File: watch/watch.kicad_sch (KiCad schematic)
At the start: 37 parts, among them IC1 MAX77659AENV+, J1 TYPE-C-31-M-12, J2 Conn_01x02_Socket, J3 Conn_ARM_JTAG_SWD_10, SW1 SW_Push, U1 nRF52840, Y1 32MHz

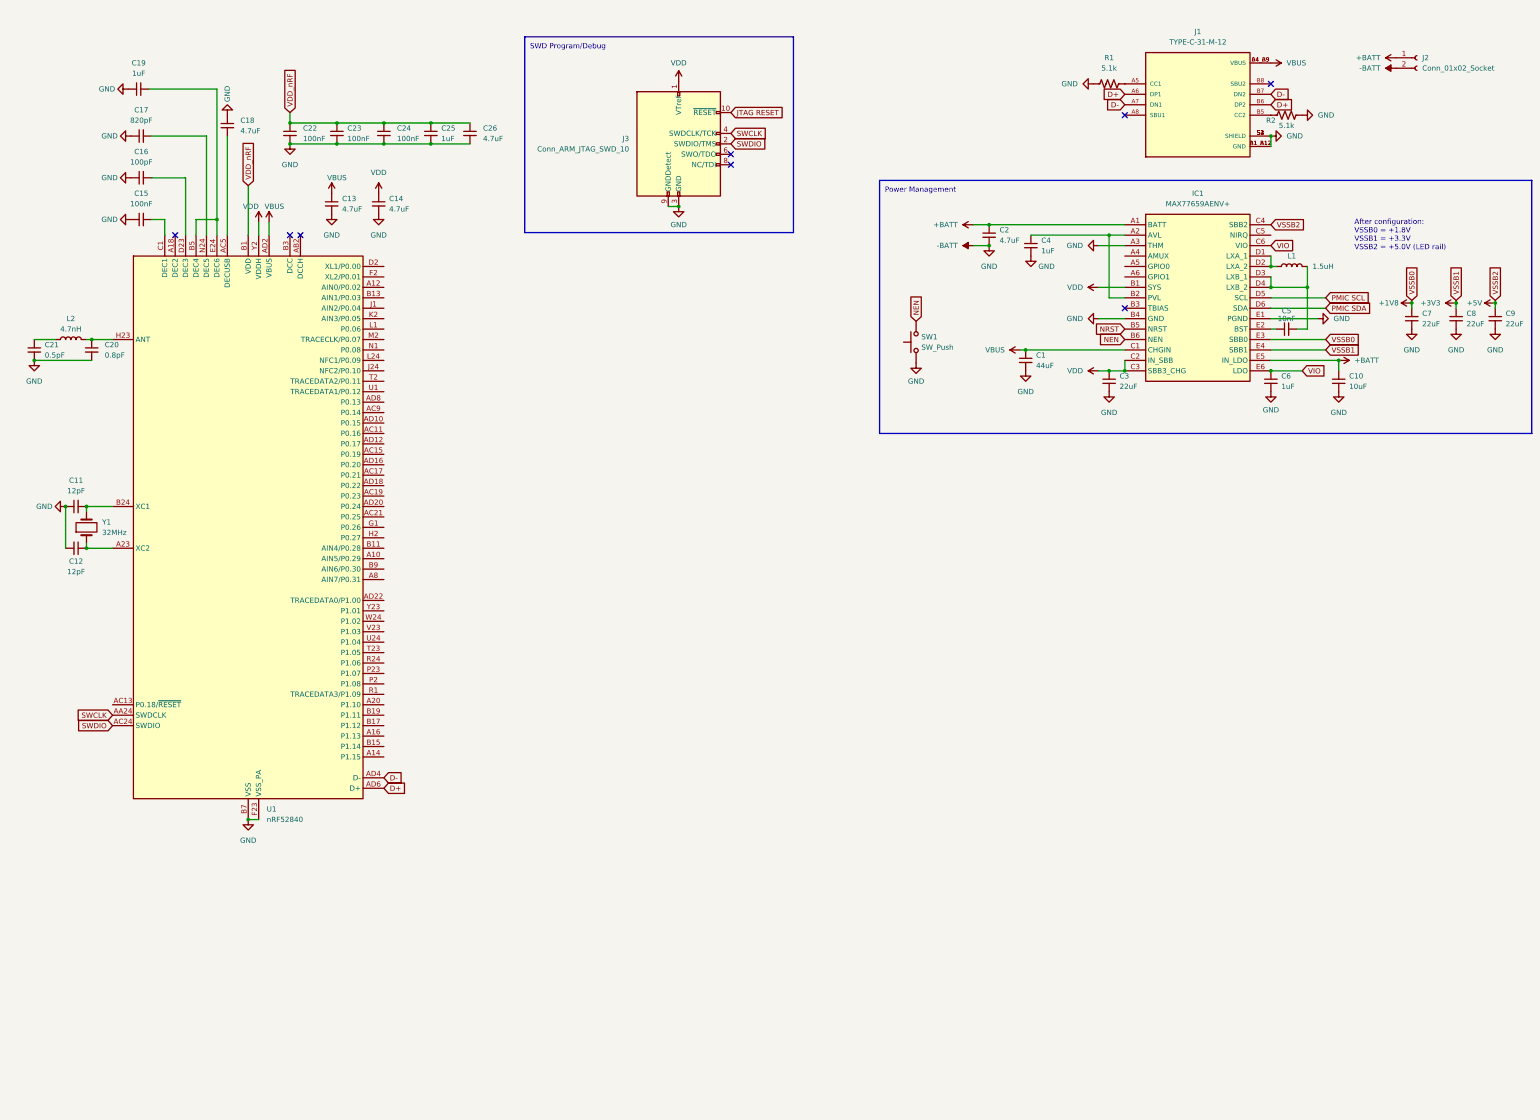
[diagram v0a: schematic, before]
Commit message: organize and add display block, going to the gym
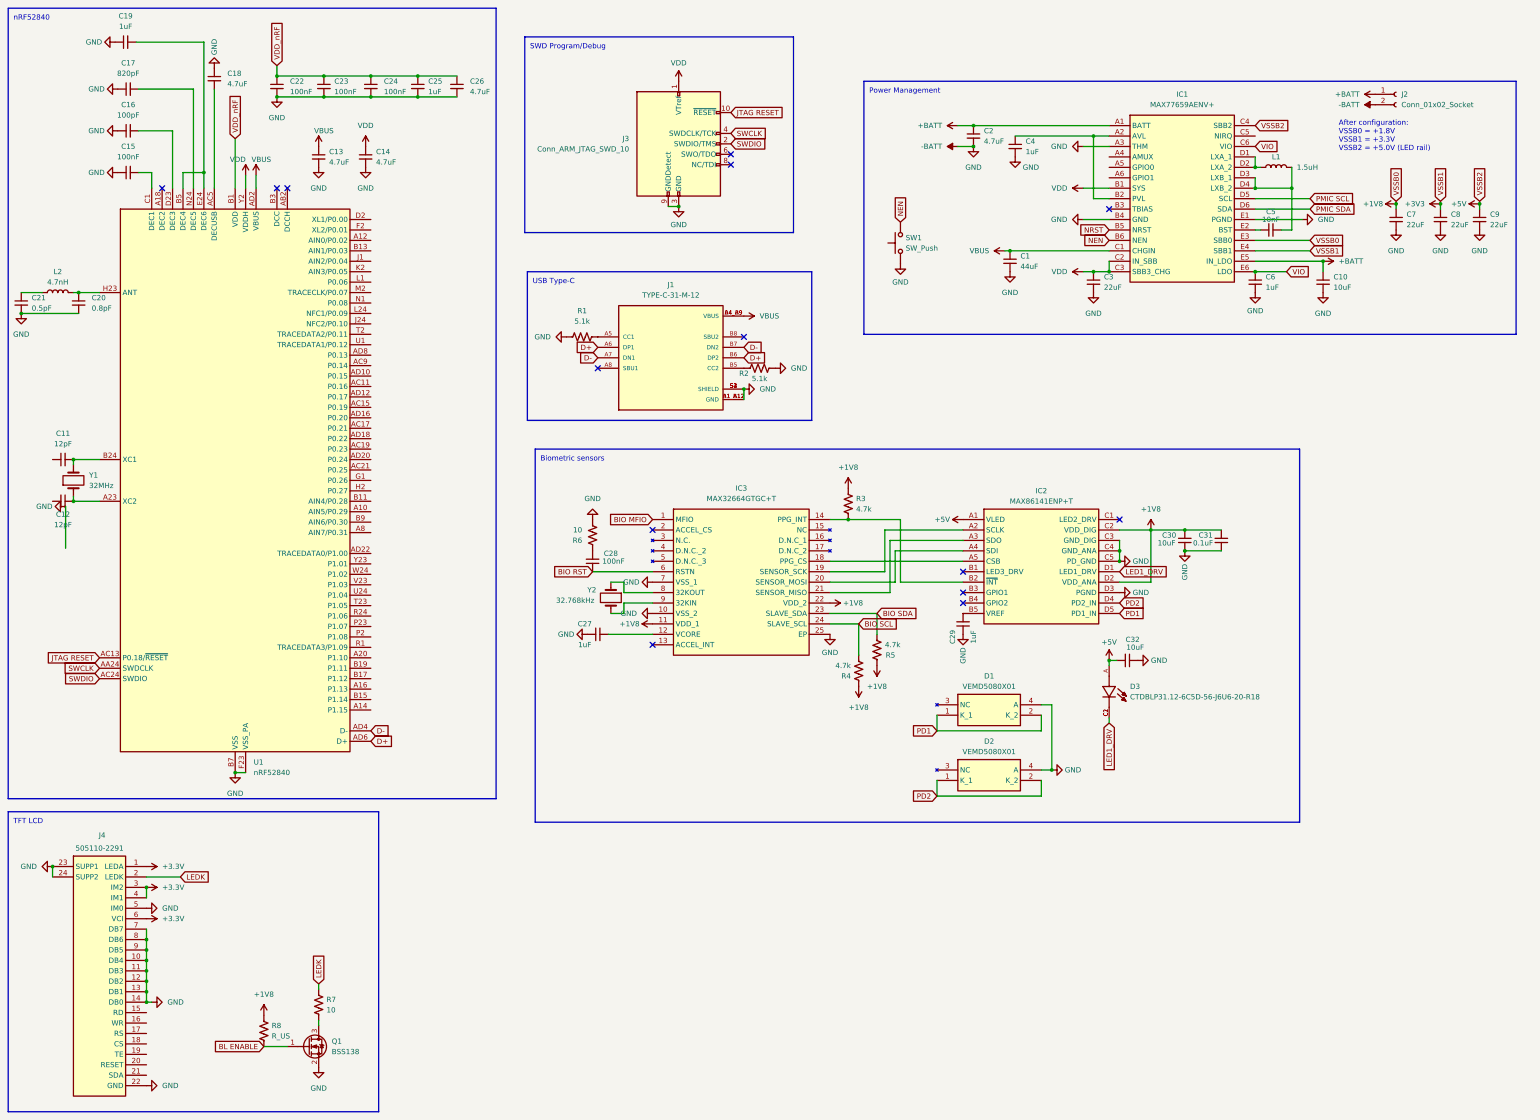
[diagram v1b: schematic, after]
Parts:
- added C27, C29: 1uF, symbol Device:C_Small
- added C28: 100nF, symbol Device:C_Small
- added C30, C32: 10uF, symbol Device:C_Small
- added C31: 0.1uF, symbol Device:C_Small
- added D1, D2: VEMD5080X01, VEMD5080X01, symbol VEMD5080X01:VEMD5080X01
- added D3: CTDBLP31.12-6C5D-56-J6U6-20-R18, LED_CTDBLP31.12-6C5D-56-J6U6-20-R18, symbol CTDBLP31.12-6C5D-56-J6U6-20-R18:CTDBLP31.12-6C5D-56-J6U6-20-R18
- added IC2: MAX86141ENP+T, BGA20C40P5X4_205X185X50, symbol MAX86141ENP+T:MAX86141ENP+T
- added IC3: MAX32664GTGC+T, MAX32664GTGC, symbol MAX32664GTGC+T:MAX32664GTGC+T
- added J4: 505110-2291, 5051102291, symbol 505110-2291:505110-2291
- added Q1: BSS138, Package_TO_SOT_SMD:SOT-23, symbol Transistor_FET:BSS138
- added R3, R4, R5: 4.7k, symbol Device:R_US
- added R6, R7: 10, symbol Device:R_US
- added R8: R_US, symbol Device:R_US
- added Y2: 32.768kHz, symbol Device:Crystal
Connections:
- net +1V8: now also C30.2, C31.2, IC2.C2 (VDD_DIG), IC2.D2 (VDD_ANA), IC3.11 (VDD_1), IC3.22 (VDD_2), R3.1, R4.1, R5.1, R8.1
- net +5V: now also C32.2, D3.A, IC2.A1 (VLED)
- net -BATT: now also C27.1, C29.1, C30.1, C31.1, C32.1, D1.4 (A), D2.4 (A), IC2.C3 (GND_DIG), IC2.C4 (GND_ANA), IC2.C5 (PD_GND), IC2.D3 (PGND), IC3.10 (VSS_2), IC3.25 (EP), IC3.7 (VSS_1), J4.10 (DB4), J4.11 (DB3), J4.12 (DB2), J4.13 (DB1), J4.14 (DB0), J4.22 (GND), J4.23 (SUPP1), J4.24 (SUPP2), J4.5 (IM0), J4.7 (DB7), J4.8 (DB6), J4.9 (DB5), Q1.2 (S), R6.1; no longer C11.1, C12.2
- net JTAG RESET: now also U1.AC13 (P0.18/~{RESET})
- new net: Q1.3 (D), R7.2
- new net: C28.2, R6.2
- new net: IC3.8 (32KOUT), Y2.1
- new net: IC3.9 (32KIN), Y2.2
- new net: C27.2, IC3.12 (VCORE)
- new net: IC2.B2 (~{INT}), IC3.14 (PPG_INT), R3.2
- new net: IC2.A5 (CSB), IC3.18 (PPG_CS)
- new net: IC2.A2 (SCLK), IC3.19 (SENSOR_SCK)
- new net: IC2.A4 (SDI), IC3.20 (SENSOR_MOSI)
- new net: IC2.A3 (SDO), IC3.21 (SENSOR_MISO)
- new net: C29.2, IC2.B5 (VREF)
- new net +3.3V: J4.1 (LEDA), J4.3 (IM2), J4.4 (IM1), J4.6 (VCI)
- new net BIO MFIO: IC3.1 (MFIO)
- new net BIO RST: C28.1, IC3.6 (RSTN)
- new net BIO SCL: IC3.24 (SLAVE_SCL), R4.2
- new net BIO SDA: IC3.23 (SLAVE_SDA), R5.2
- new net BL ENABLE: Q1.1 (G), R8.2
- new net LED1_DRV: D3.C1, D3.C2, IC2.D1 (LED1_DRV)
- new net LEDK: J4.2 (LEDK), R7.1
- new net PD1: D1.1 (K_1), D1.2 (K_2), IC2.D5 (PD1_IN)
- new net PD2: D2.1 (K_1), D2.2 (K_2), IC2.D4 (PD2_IN)
- no-connect marks 8 -> 14
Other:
- note added: "Biometric sensors"
- note added: "TFT LCD"
- note added: "USB Type-C"
- note added: "nRF52840"
- moved on the sheet: C1, C10, C11, C12, C13, C14, C15, C16, C17, C18, C19, C2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
